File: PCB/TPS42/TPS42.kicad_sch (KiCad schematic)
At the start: 79 parts, among them J1 PJ-320A, J11 Conn_01x06, J13 Conn_01x09, J14 FH12-10S-0.5SH, J2 Conn_01x09, J3 TP Sensor Module, J4 TP Module, J6 OLED, J7 TrackPoint, J8 Battery, J9 TP Sensor Module, SW1 SW_DPST_x2, SW2 Reset, SW3 Reset, U1 ProMicro, U11 Hole, U12 Hole, U14 ProMicro, U2 Hole, U3 Hole, U4 Hole, U5 Hole, U7 Hole, U8 Hole, U9 Hole

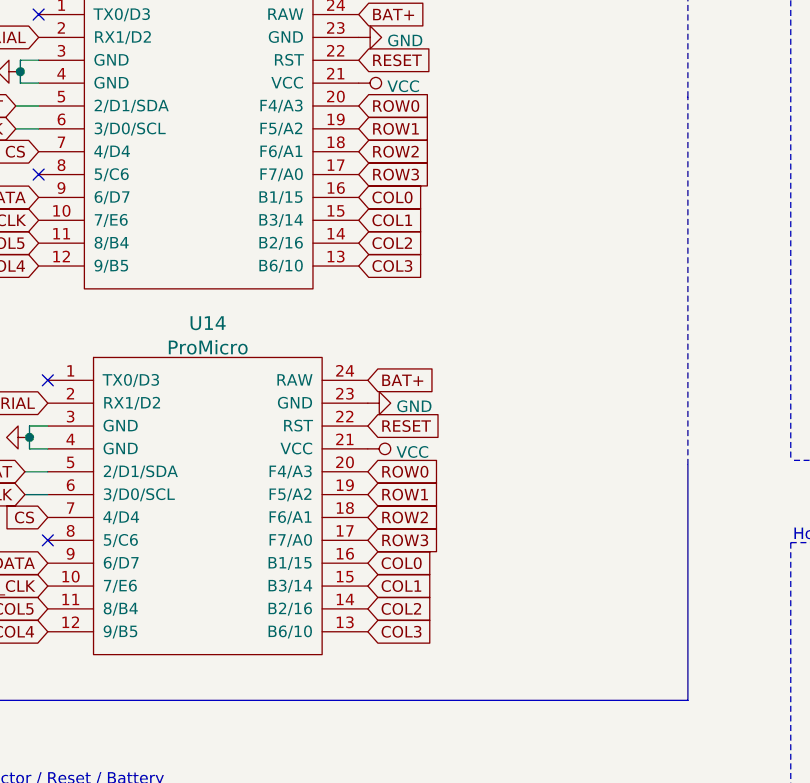
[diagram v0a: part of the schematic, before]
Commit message: started routing
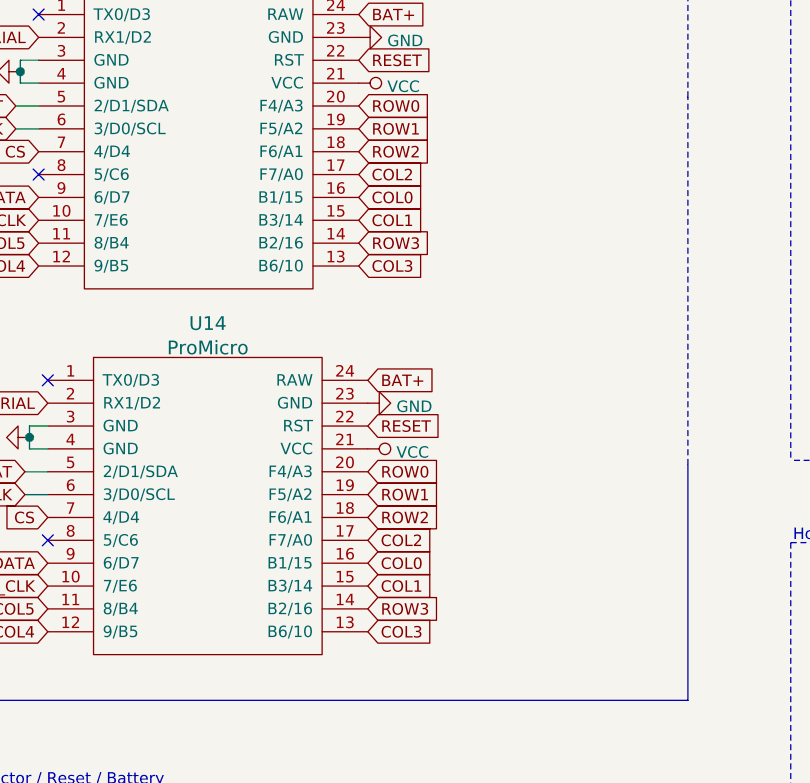
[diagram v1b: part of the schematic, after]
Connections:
- net COL2: now also U1.17 (F7/A0), U14.17 (F7/A0); no longer U1.14 (B2/16), U14.14 (B2/16)
- net ROW3: now also U1.14 (B2/16), U14.14 (B2/16); no longer U1.17 (F7/A0), U14.17 (F7/A0)
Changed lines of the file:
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@@
-    )
-  )
-  (global_label "COL2" (shape input) (at 66.294 93.472 0) (fields_autoplaced)
-    (effects (font (size 1.27 1.27)) (justify left))
-    (property "Intersheet References" "${INTERSHEET_REFS}" (id 0) (at 73.5452 93.3926 0)
-      (effects (font (size 1.27 1.27)) (justify left) hide)
     )
   )
@@
     )
   )
-  (global_label "ROW3" (shape input) (at 66.294 85.852 0) (fields_autoplaced)
-    (effects (font (size 1.27 1.27)) (justify left))
-    (property "Intersheet References" "${INTERSHEET_REFS}" (id 0) (at 73.9685 85.7726 0)
-      (effects (font (size 1.27 1.27)) (justify left) hide)
-    )
-  )
   (global_label "ROW0" (shape input) (at 133.35 31.242 180) (fields_autoplaced)
     (effects (font (size 1.27 1.27)) (justify right))
@@
     )
   )
+  (global_label "ROW3" (shape input) (at 65.278 52.832 0) (fields_autoplaced)
+    (effects (font (size 1.27 1.27)) (justify left))
+    (property "Intersheet References" "${INTERSHEET_REFS}" (id 0) (at 72.9525 52.7526 0)
+      (effects (font (size 1.27 1.27)) (justify left) hide)
+    )
+  )
   (global_label "CLK" (shape input) (at 28.194 80.772 180) (fields_autoplaced)
     (effects (font (size 1.27 1.27)) (justify right))
@@
     )
   )
-  (global_label "COL2" (shape input) (at 65.278 52.832 0) (fields_autoplaced)
-    (effects (font (size 1.27 1.27)) (justify left))
-    (property "Intersheet References" "${INTERSHEET_REFS}" (id 0) (at 72.5292 52.7526 0)
-      (effects (font (size 1.27 1.27)) (justify left) hide)
-    )
-  )
   (global_label "TP_CLK" (shape input) (at 38.354 163.576 180) (fields_autoplaced)
     (effects (font (size 1.27 1.27)) (justify right))
@@
     )
   )
-  (global_label "ROW3" (shape input) (at 65.278 45.212 0) (fields_autoplaced)
-    (effects (font (size 1.27 1.27)) (justify left))
-    (property "Intersheet References" "${INTERSHEET_REFS}" (id 0) (at 72.9525 45.1326 0)
-      (effects (font (size 1.27 1.27)) (justify left) hide)
-    )
-  )
   (global_label "COL0" (shape input) (at 65.278 47.752 0) (fields_autoplaced)
     (effects (font (size 1.27 1.27)) (justify left))
@@
     )
   )
+  (global_label "COL2" (shape input) (at 66.294 85.852 0) (fields_autoplaced)
+    (effects (font (size 1.27 1.27)) (justify left))
+    (property "Intersheet References" "${INTERSHEET_REFS}" (id 0) (at 73.5452 85.7726 0)
+      (effects (font (size 1.27 1.27)) (justify left) hide)
+    )
+  )
+  (global_label "COL2" (shape input) (at 65.278 45.212 0) (fields_autoplaced)
+    (effects (font (size 1.27 1.27)) (justify left))
+    (property "Intersheet References" "${INTERSHEET_REFS}" (id 0) (at 72.5292 45.1326 0)
+      (effects (font (size 1.27 1.27)) (justify left) hide)
+    )
+  )
   (global_label "COL0" (shape input) (at 66.294 88.392 0) (fields_autoplaced)
     (effects (font (size 1.27 1.27)) (justify left))
@@
     )
   )
+  (global_label "ROW3" (shape input) (at 66.294 93.472 0) (fields_autoplaced)
+    (effects (font (size 1.27 1.27)) (justify left))
+    (property "Intersheet References" "${INTERSHEET_REFS}" (id 0) (at 73.9685 93.3926 0)
+      (effects (font (size 1.27 1.27)) (justify left) hide)
+    )
+  )
